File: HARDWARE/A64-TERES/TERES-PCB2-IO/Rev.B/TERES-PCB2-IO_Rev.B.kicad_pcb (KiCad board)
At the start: 2 copper layers, 25.5 x 73.5 mm, 46 parts, among them J1 EZ-PJ-3510A-W-H, P1 USB-3.5mm(TERES), P2 CONN_01X40, P3 CONN_01X02, P4 CONN_01X02

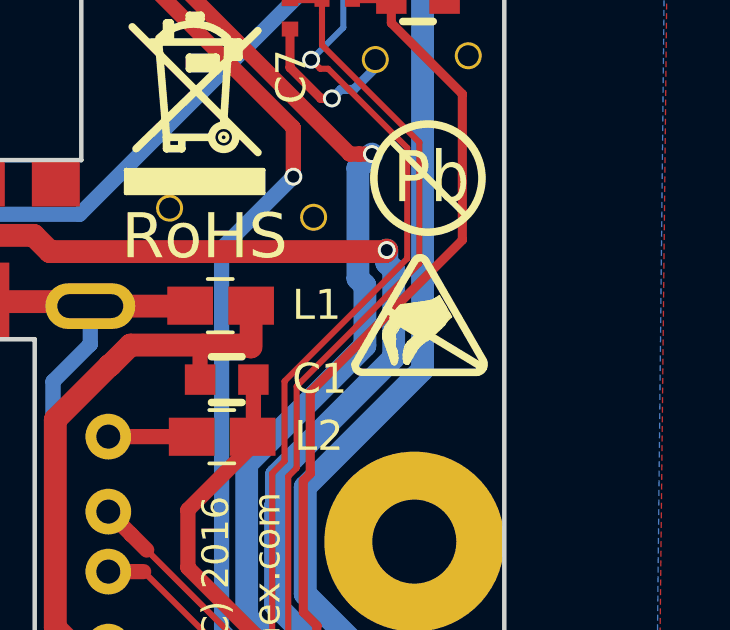
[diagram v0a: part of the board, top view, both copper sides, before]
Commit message: Update projects using KiCAD 6.0.7
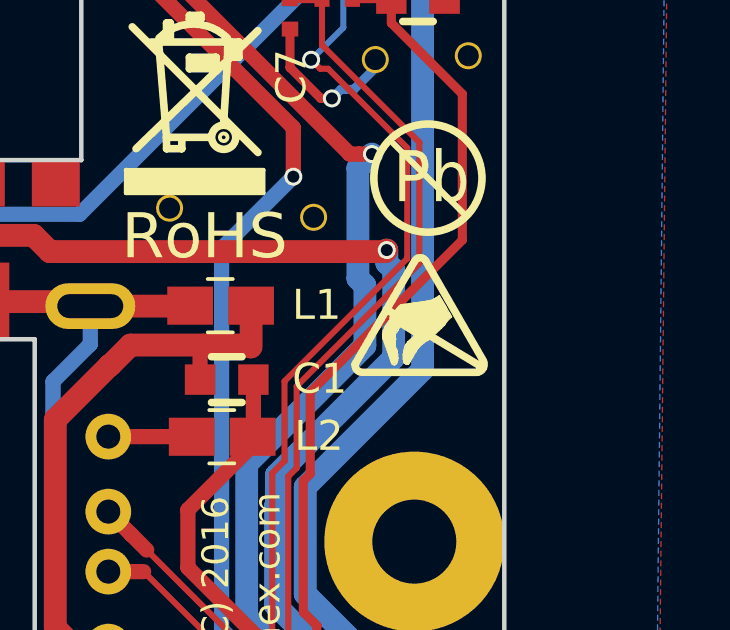
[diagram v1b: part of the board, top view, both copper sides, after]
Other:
- net class Default removed
